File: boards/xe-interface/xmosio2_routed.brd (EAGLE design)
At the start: 116.8 x 100 mm, 121 parts, among them IC1 IDTQS3245QSOP20, IC2 IDTQS3245QSOP20, IC3 IDTQS3245QSOP20, IC4 IDTQS3245QSOP20, IC5 IDTQS3245QSOP20, U1 24 MHz Osc. (F535L-24), X1 0446200002

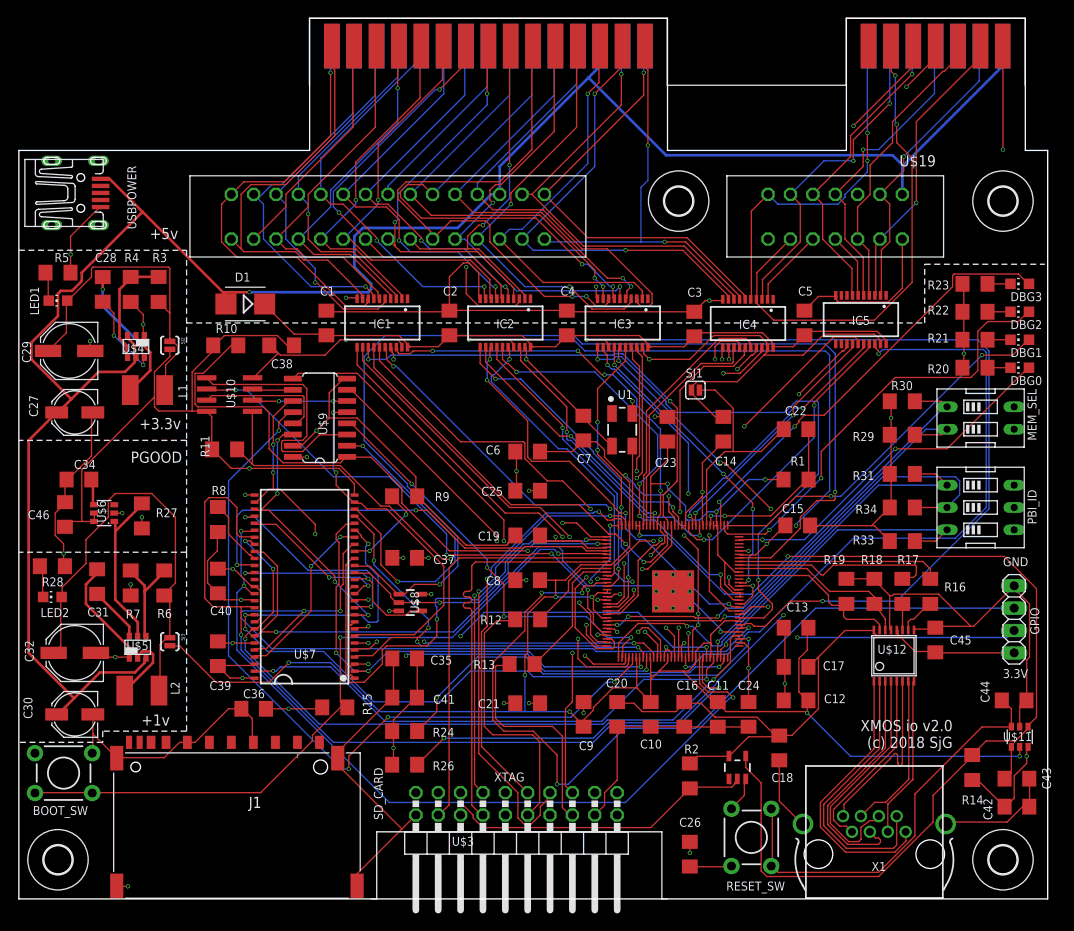
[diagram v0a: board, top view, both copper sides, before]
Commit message: Add a new progress post
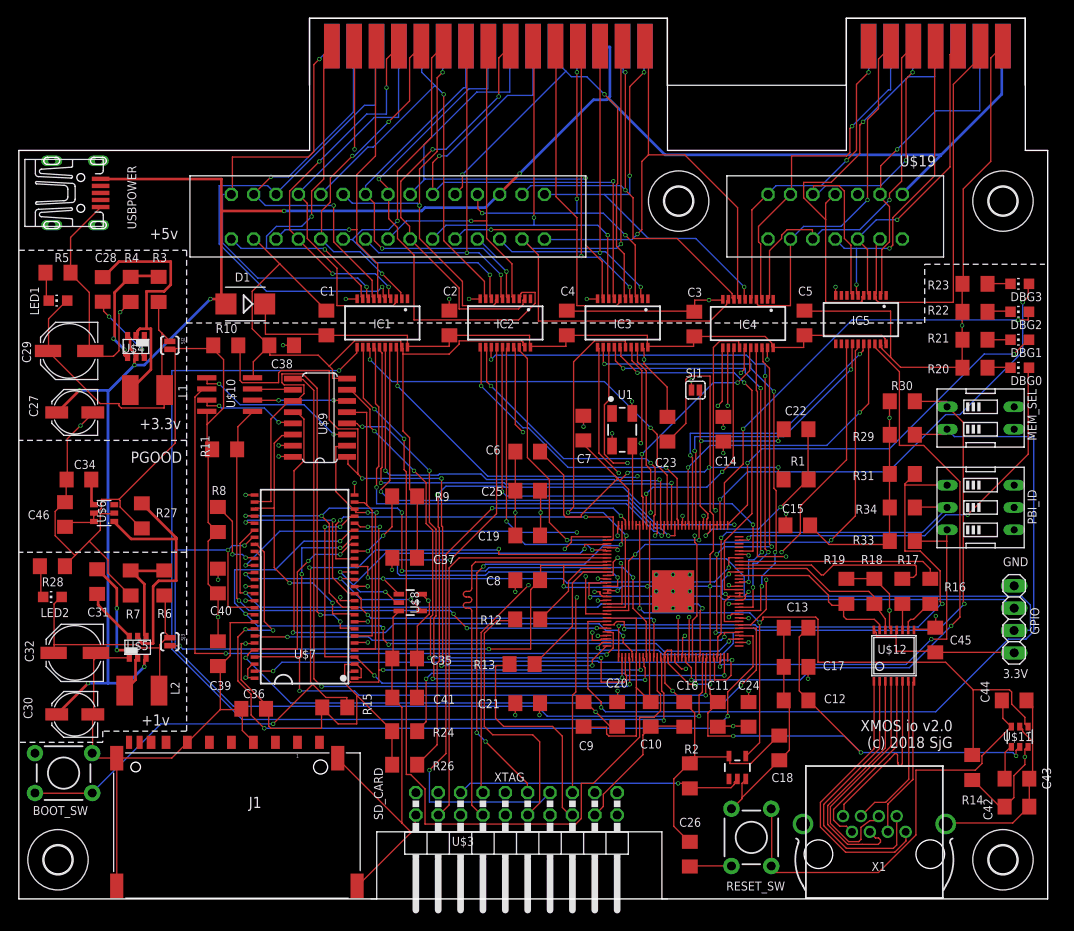
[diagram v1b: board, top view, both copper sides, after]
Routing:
- net !SD_CAS!: track 128.9 -> 49.6 mm, vias 2 -> 3
- net X_RD4: track 54.6 -> 120.7 mm
- net X_D0: track 101.4 -> 43.8 mm
- net VCCINT: track 254.1 -> 305.2 mm, vias 11 -> 16
- net N$34: track 51.6 -> 102.2 mm
- net !X_S4!: track 51.9 -> 99.3 mm
- net N$37: track 97.4 -> 52.5 mm, vias 3 -> 1
- net X_D2: track 82.4 -> 43.5 mm, vias 3 -> 2
- net !RESET!: track 122.3 -> 87.7 mm
- net VCCIO: track 272.5 -> 244.3 mm, vias 24 -> 30
- net X_A8: track 33.7 -> 61.6 mm
- net SD_ADQ8: track 93.0 -> 68.3 mm, vias 3 -> 2
- net X_D1: track 61.1 -> 39.3 mm
- net SD_ADQ5/QS_D3: track 88.7 -> 67.7 mm, vias 4 -> 2
- net QSPI_CLK: track 60.3 -> 81.2 mm, vias 4 -> 2
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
